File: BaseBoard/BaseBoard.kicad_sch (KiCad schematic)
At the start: 22 parts, among them J1 OHIS RJ45, J2 Radio Board, J3 Dynamic/Electret, J6 Speaker Input Config

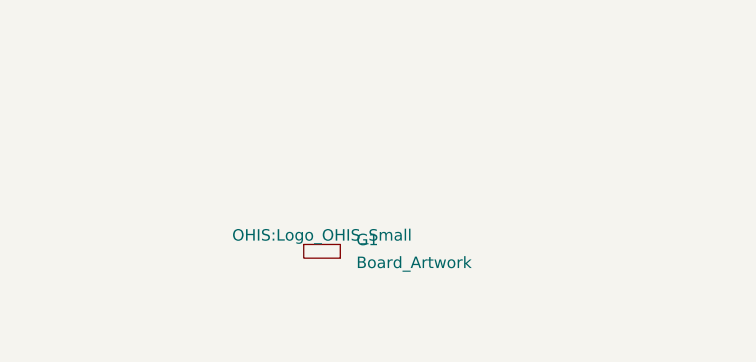
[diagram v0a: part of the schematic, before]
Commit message: Happy with BaseBoard and Icom-RJ45. Working on Icom-GX16 #1
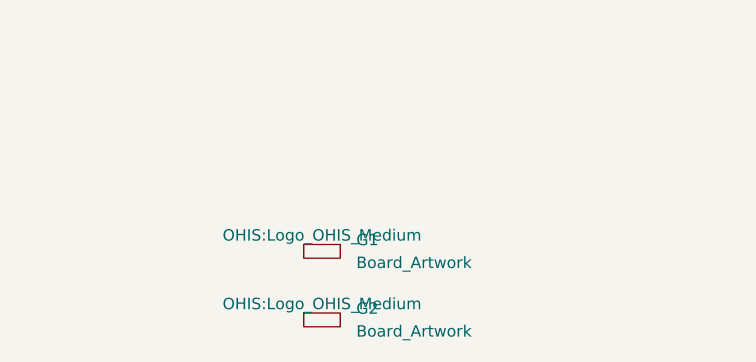
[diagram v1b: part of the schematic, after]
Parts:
- added G2: Board_Artwork, OHIS:Logo_OHIS_Medium, symbol Smitty:Board_Artwork
- G1: footprint OHIS:Logo_OHIS_Small -> OHIS:Logo_OHIS_Medium
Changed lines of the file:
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@@
+	)
+	(symbol
+		(lib_id "Smitty:Board_Artwork")
+		(at 83.82 168.91 0)
+		(unit 1)
+		(exclude_from_sim no)
+		(in_bom no)
+		(on_board yes)
+		(dnp no)
+		(fields_autoplaced yes)
+		(property "Reference" "G2"
+			(at 87.63 169.4179 0)
+			(effects
+				(font
+					(size 1.27 1.27)
+				)
+				(justify left)
+			)
+		)
+		(property "Value" "Board_Artwork"
+			(at 87.63 171.9579 0)
+			(effects
+				(font
+					(size 1.27 1.27)
+				)
+				(justify left)
+			)
+		)
+		(property "Footprint" "OHIS:Logo_OHIS_Medium"
+			(at 83.82 168.91 0)
+			(effects
+				(font
+					(size 1.27 1.27)
+				)
+			)
+		)
+		(property "Datasheet" ""
+			(at 83.82 168.91 0)
+			(effects
+				(font
+					(size 1.27 1.27)
+				)
+				(hide yes)
+			)
+		)
+		(property "Description" ""
+			(at 83.82 168.91 0)
+			(effects
+				(font
+					(size 1.27 1.27)
+				)
+				(hide yes)
+			)
+		)
+		(instances
+			(project "BaseBoard"
+				(path "/6a3924fa-c381-477c-bc5e-4effe098c460"
+					(reference "G2")
+					(unit 1)
+				)
+			)
+		)
 	)
 	(symbol
@@
 			)
 		)
-		(property "Footprint" "OHIS:Logo_OHIS_Small"
+		(property "Footprint" "OHIS:Logo_OHIS_Medium"
 			(at 83.82 161.29 0)
 			(effects

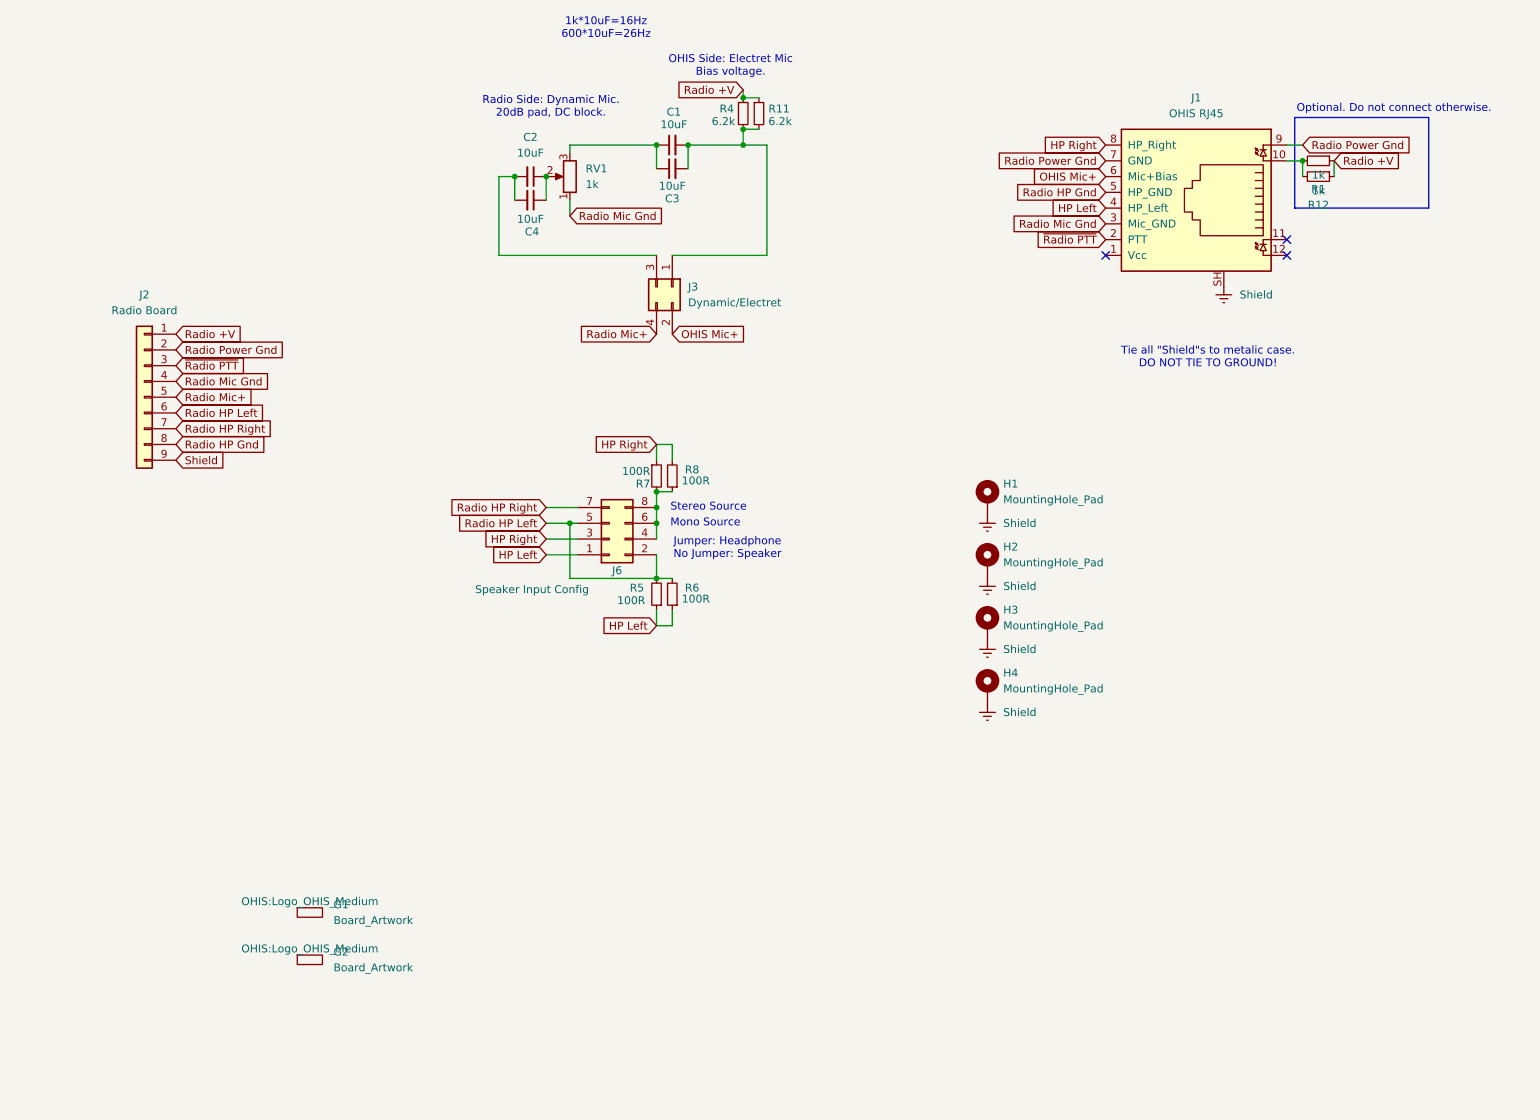
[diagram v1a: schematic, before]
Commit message: Updated BOM parts, among other things. Sorry, it's been a while. #1
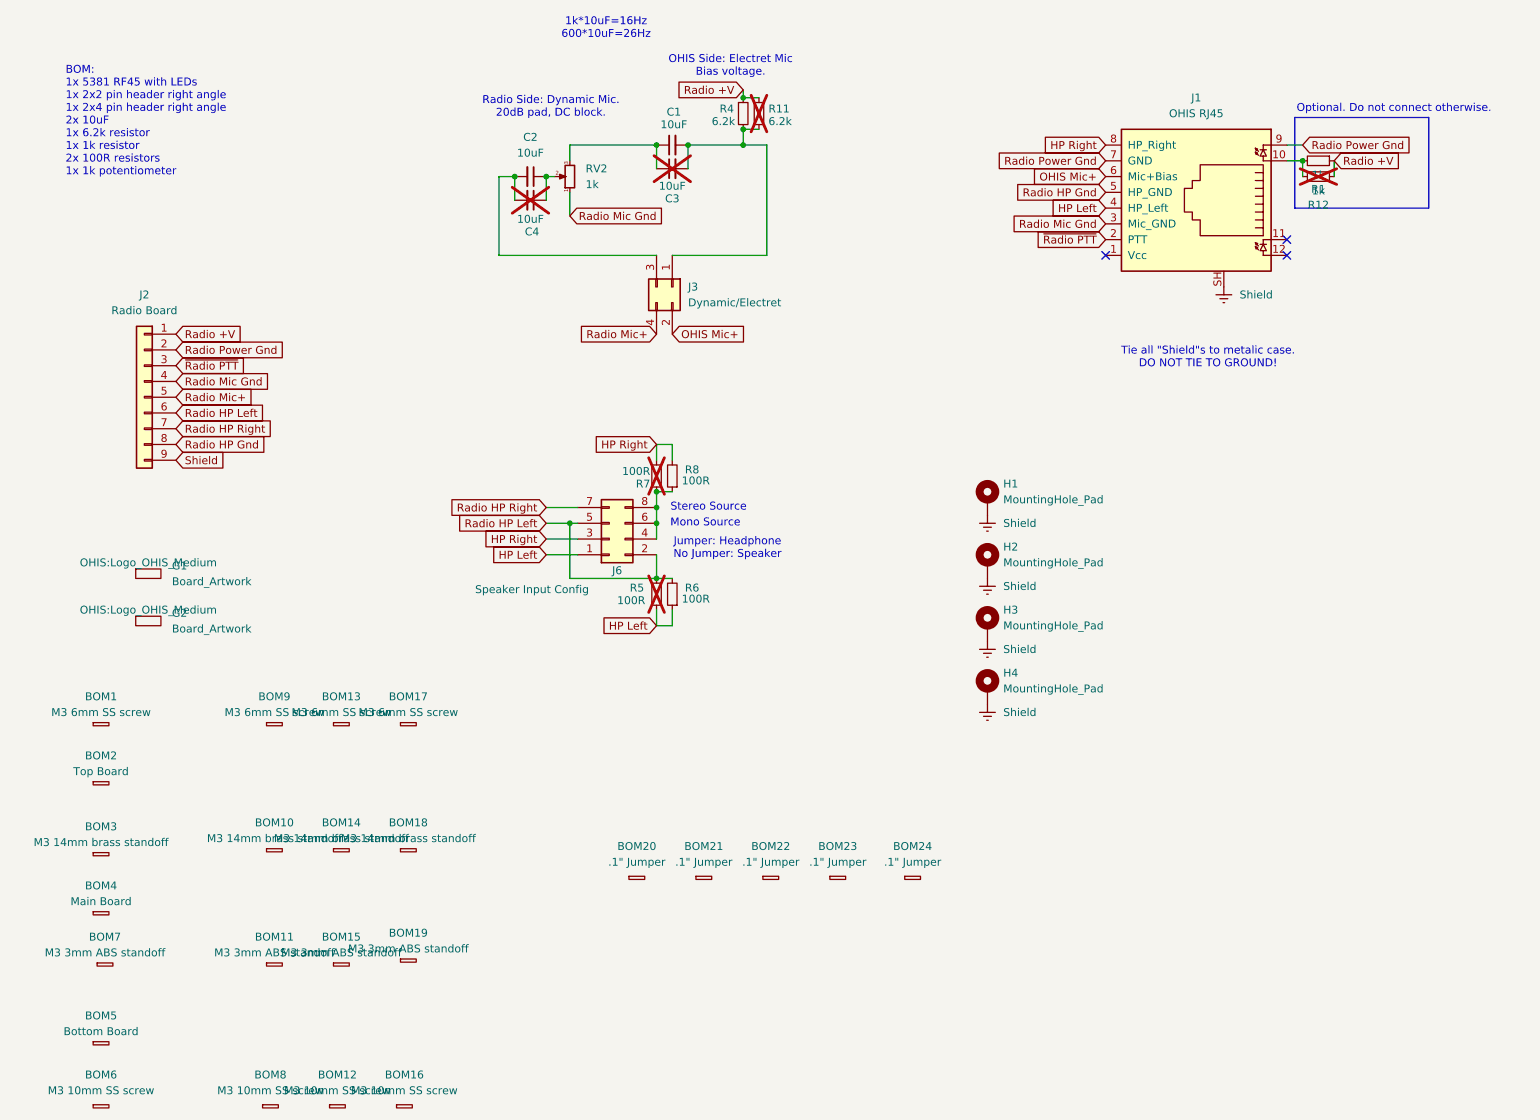
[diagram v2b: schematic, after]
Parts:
- removed RV1: 1k, Potentiometer_THT:Potentiometer_Piher_PT-6-H_Horizontal, symbol Device:R_Potentiometer
- added BOM1, BOM13, BOM17, BOM9: M3 6mm SS screw, Libraries:BOM_Item, symbol smitty:BOM_Item
- added BOM10, BOM14, BOM18, BOM3: M3 14mm brass standoff, Libraries:BOM_Item, symbol smitty:BOM_Item
- added BOM11, BOM15, BOM19, BOM7: M3 3mm ABS standoff, Libraries:BOM_Item, symbol smitty:BOM_Item
- added BOM12, BOM16, BOM6, BOM8: M3 10mm SS screw, Libraries:BOM_Item, symbol smitty:BOM_Item
- added BOM2: Top Board, Libraries:BOM_Item, symbol smitty:BOM_Item
- added BOM20, BOM21, BOM22, BOM23, BOM24: .1" Jumper, Libraries:BOM_Item, symbol smitty:BOM_Item
- added BOM4: Main Board, Libraries:BOM_Item, symbol smitty:BOM_Item
- added BOM5: Bottom Board, Libraries:BOM_Item, symbol smitty:BOM_Item
- added RV2: 1k, Potentiometer_THT:Potentiometer_Piher_PT-6-H_Horizontal, symbol Device:R_Potentiometer_Small
- C1, C2: Link (none) -> https://www.mouser.com/ProductDetail/TDK/FG28X5R1E106MRT06?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; Manufacturer (none) -> TDK; Part Number (none) -> FG28X5R1E106MRT06; Z0 Buy in Qty (none) -> 200; Z1 Cost to buy (none) -> =32.40
- C3, C4, R11, R12, R5, R7: now not fitted; now left out of the parts list
- J1: Link (none) -> https://www.mouser.com/ProductDetail/523-RJHSE-5380; Manufacturer (none) -> Amphenol; Part Number (none) -> RJHSE-5381; Z0 Buy in Qty (none) -> 120; Z1 Cost to buy (none) -> =127.20; Z2 Cost per part (none) -> =IFERROR(OFFSET(INDIRECT(CELL("Address")), 0, -1)/OFFSET(IN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; Z3 Cost per Qty (none) -> =OFFSET(INDIRECT(CELL("Address")), 0, -1)*INDIRECT(ADDRESS(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
- J3, J6: Link (none) -> https://www.ebay.com/itm/181918596973; Manufacturer (none) -> Generic; Part Number (none) -> .1" 3x40 right angle 2.54mm Pin Header; Z0 Buy in Qty (none) -> 40; Z1 Cost to buy (none) -> 2.49; Z2 Cost per part (none) -> =IFERROR(OFFSET(INDIRECT(CELL("Address")), 0, -1)/OFFSET(IN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; Z3 Cost per Qty (none) -> =OFFSET(INDIRECT(CELL("Address")), 0, -1)*INDIRECT(ADDRESS(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
- R1: Link (none) -> https://www.mouser.com/ProductDetail/YAGEO/CFR-12JB-52-1K?q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; Manufacturer (none) -> YAGEO; Part Number (none) -> CFR-12JB-52-1K; Z0 Buy in Qty (none) -> 100; Z1 Cost to buy (none) -> 2.80; Z2 Cost per part (none) -> =IFERROR(OFFSET(INDIRECT(CELL("Address")), 0, -1)/OFFSET(IN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; Z3 Cost per Qty (none) -> =OFFSET(INDIRECT(CELL("Address")), 0, -1)*INDIRECT(ADDRESS(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
- R4: Link (none) -> https://www.mouser.com/ProductDetail/YAGEO/CFR-12JB-52-6K2?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; Manufacturer (none) -> YAGEO; Part Number (none) -> CFR-12JB-52-6K2; Z0 Buy in Qty (none) -> 100; Z1 Cost to buy (none) -> 1.90
- R6, R8: Link (none) -> https://www.mouser.com/ProductDetail/YAGEO/CFR-12JB-52-100R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; Manufacturer (none) -> YAGEO; Part Number (none) -> CFR-12JB-52-100R; Z0 Buy in Qty (none) -> 100; Z1 Cost to buy (none) -> 2.80; Z2 Cost per part (none) -> =IFERROR(OFFSET(INDIRECT(CELL("Address")), 0, -1)/OFFSET(IN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; Z3 Cost per Qty (none) -> =OFFSET(INDIRECT(CELL("Address")), 0, -1)*INDIRECT(ADDRESS(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
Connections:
- net Radio Mic Gnd: now also RV2.1
- net at C2.1, C4.1: now also RV2.2
- net at C1.1, C3.1: now also RV2.3
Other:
- note added: "BOM: 1x 5381 RF45 with LEDs 1x 2x2 pin header right angle 1x 2x4 pin header right angle 2x 10uF 1x 6.2k resistor 1x 1k resistor 2x 100R resistors 1x 1k potentiometer"
- moved on the sheet: G1, G2
